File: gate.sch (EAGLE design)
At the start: 20 parts, among them IC1 MAX3232CSE, IC2 LM386M-1, J1 RJ11-2X, X1 MINI-USB-SCHIELD-32005-301

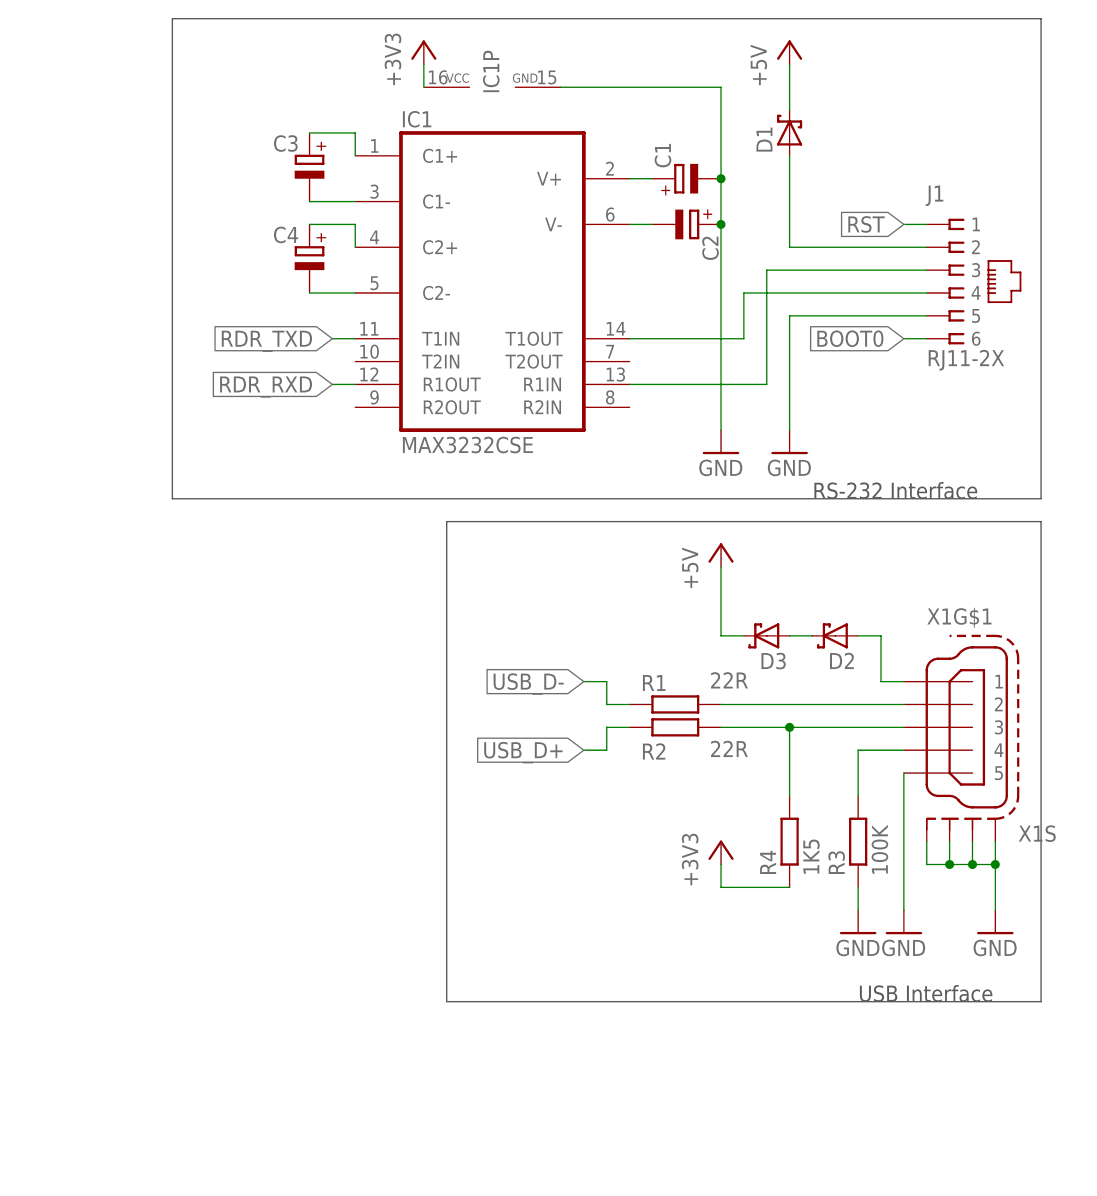
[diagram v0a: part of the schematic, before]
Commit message: Minor mid-review fixes
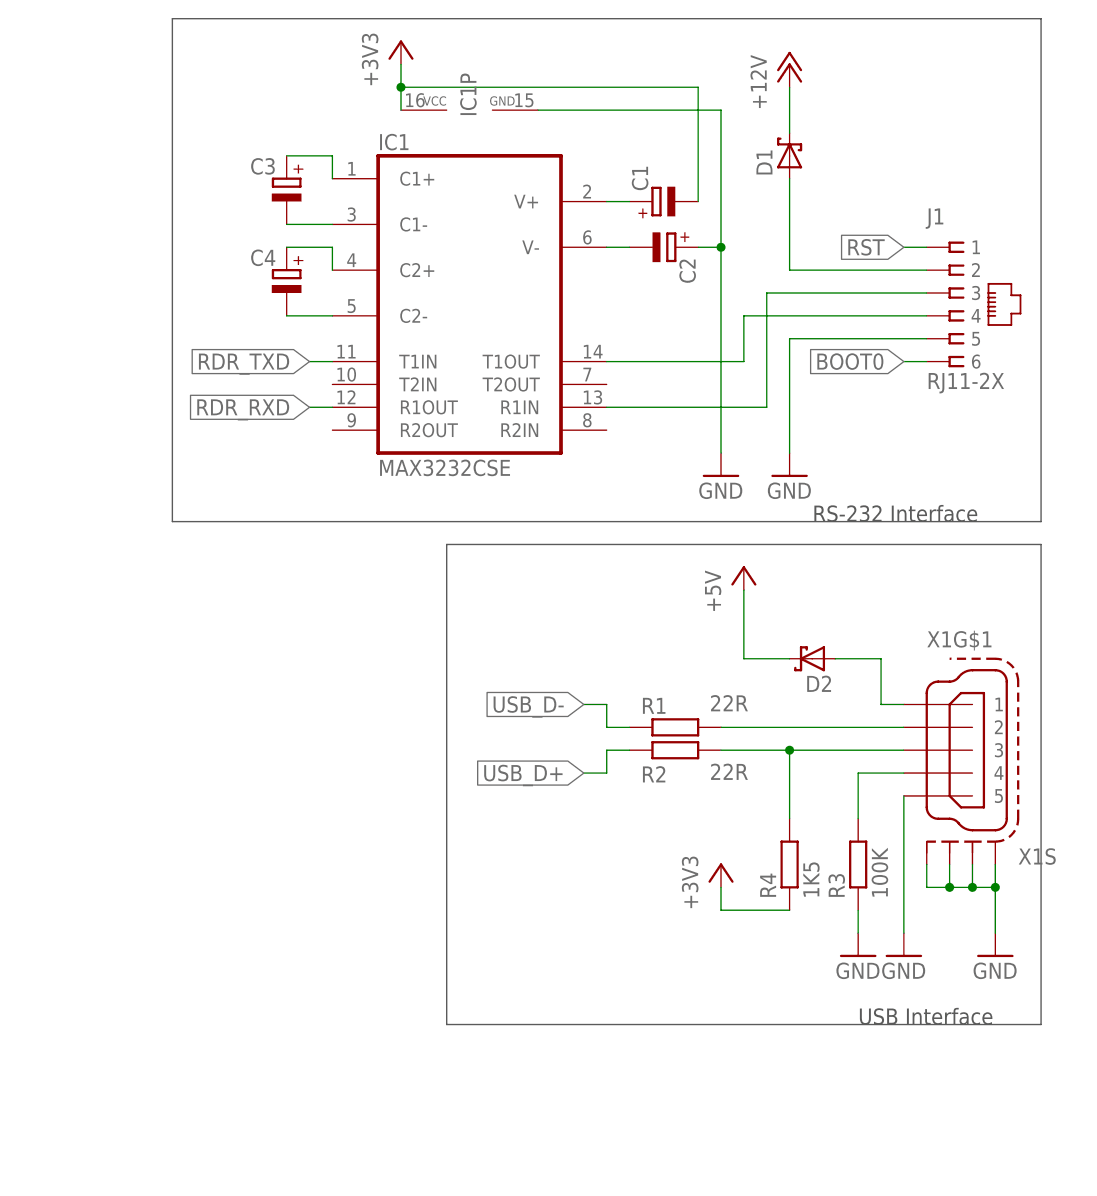
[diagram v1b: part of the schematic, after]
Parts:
- removed D3: (no value), diode:SCHOTTKY-DIODESMD
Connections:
- removed net N$10: D2.C, D3.A
- new net +12V: D1.C
- net +3V3: now also C1.-
- net +5V: now also D2.C; no longer D1.C, D3.C
- net GND: no longer C1.-
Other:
- moved on the sheet: C1, C2, C3, C4, D1, D2, IC1, IC1P, J1, R1, R2, R3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
